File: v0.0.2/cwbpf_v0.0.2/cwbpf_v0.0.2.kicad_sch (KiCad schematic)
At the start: 9 parts, among them J1 AudioJack4, U1 PCM5102A, U2 PCM1808PWR

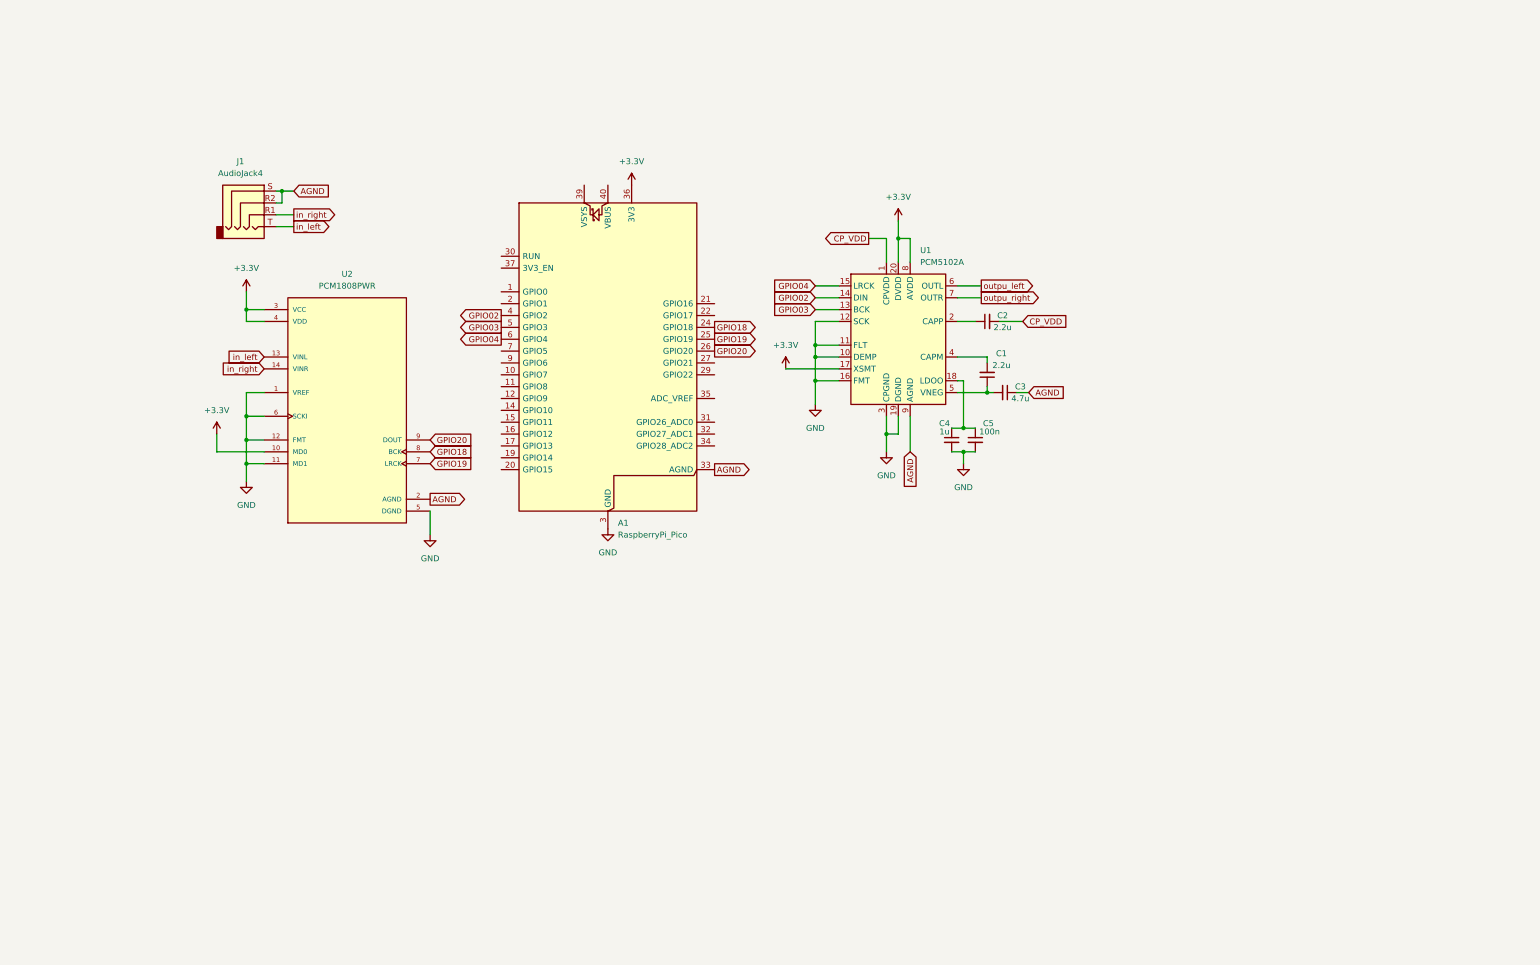
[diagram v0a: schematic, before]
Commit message: tmp
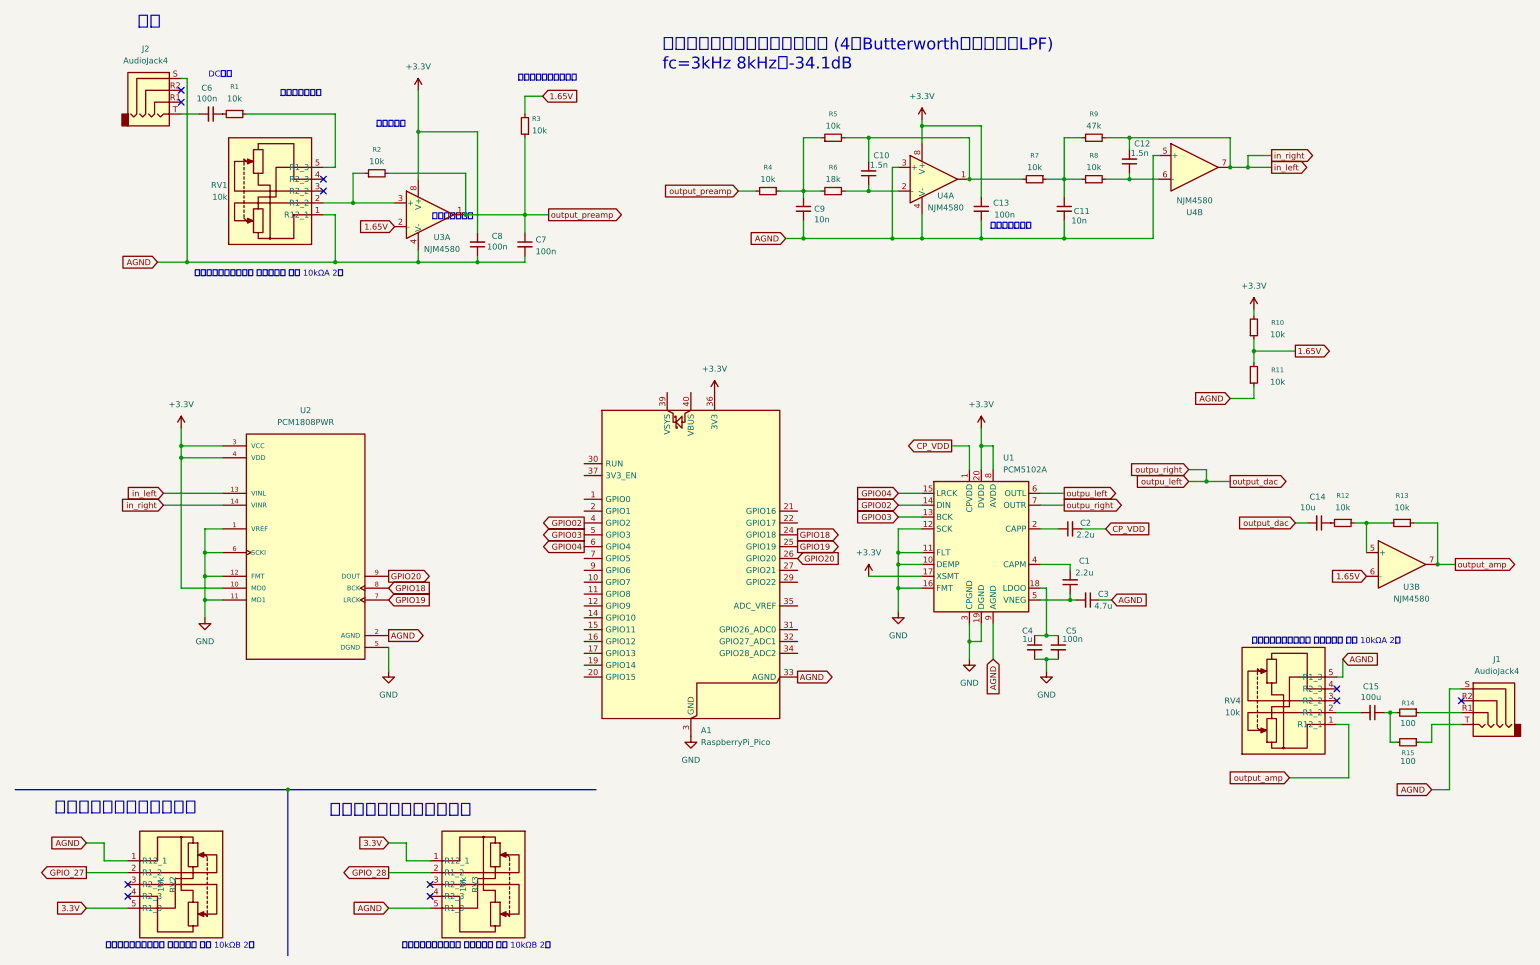
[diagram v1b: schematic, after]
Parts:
- added C10, C12: 1.5n, Capacitor_THT:C_Disc_D7.0mm_W2.5mm_P5.00mm, symbol Device:C_Small
- added C11, C9: 10n, Capacitor_THT:C_Disc_D7.0mm_W2.5mm_P5.00mm, symbol Device:C_Small
- added C13, C6, C7, C8: 100n, Capacitor_THT:C_Disc_D7.5mm_W2.5mm_P5.00mm, symbol Device:C_Small
- added C14: 10u, Capacitor_THT:CP_Radial_D5.0mm_P2.00mm, symbol Device:C_Small
- added C15: 100u, Capacitor_THT:CP_Radial_D8.0mm_P3.50mm, symbol Device:C_Small
- added J2: AudioJack4, Connector_Audio:Jack_3.5mm_PJ320E_Horizontal, symbol Connector_Audio:AudioJack4
- added R1, R10, R11, R12, R13, R2, R3, R4, R5, R7, R8: 10k, Resistor_THT:R_Axial_DIN0204_L3.6mm_D1.6mm_P5.08mm_Horizontal, symbol Device:R_Small
- added R14, R15: 100, Resistor_THT:R_Axial_DIN0204_L3.6mm_D1.6mm_P5.08mm_Horizontal, symbol Device:R_Small
- added R6: 18k, Resistor_THT:R_Axial_DIN0204_L3.6mm_D1.6mm_P5.08mm_Horizontal, symbol Device:R_Small
- added R9: 47k, Resistor_THT:R_Axial_DIN0204_L3.6mm_D1.6mm_P5.08mm_Horizontal, symbol Device:R_Small
- added RV1, RV2, RV3, RV4: 10k, Library:基板取付用ボリューム つまみ付き 薄型 10kΩ 2連, symbol Library:基板取付用ボリューム つまみ付き 薄型 2連
- added U3, U4: NJM4580, Package_SIP:SIP-8_19x3mm_P2.54mm, symbol Amplifier_Operational:NJM4580
- J1: footprint (none) -> Connector_Audio:Jack_3.5mm_PJ320E_Horizontal
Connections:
- net outpu_right is gone; now on net outpu_left: U1.7 (OUTR)
- net +3.3V: now also C13.1, C8.2, R10.2, U3.8 (V+), U4.8 (V+)
- net AGND: now also C11.2, C13.2, C7.2, C8.1, C9.2, J2.S, R11.1, RV1.1 (R12_1), RV2.1 (R12_1), RV3.5 (R1_3), RV4.5 (R1_3), U3.4 (V-), U4.3 (+), U4.4 (V-), U4.5 (+); no longer J1.R2
- net in_left: now also U2.14 (VINR), C12.2, R9.2, U4.7; no longer J1.T
- net outpu_left: now also C14.2
- net in_right: no longer names the net of J1.R1
- net in_right: now also R14.1; no longer U2.14 (VINR)
- new net: R12.1, R13.2, U3.5 (+)
- new net: J1.T, R15.1
- new net: C14.1, R12.2
- new net: C11.1, R7.1, R8.1, R9.1
- new net: C15.1, R14.2, R15.2
- new net: C15.2, RV4.2 (R1_2)
- new net: C9.1, R4.1, R5.1, R6.1
- new net: R2.1, RV1.2 (R1_2), U3.3 (+)
- new net: C10.2, R5.2, R7.2, U4.1
- new net: C6.2, J2.T
- new net: C10.1, R6.2, U4.2 (-)
- new net: C12.1, R8.2, U4.6 (-)
- new net: R1.1, RV1.5 (R1_3)
- new net: C6.1, R1.2
- new net 1.65V: R10.1, R11.2, R3.2, U3.2 (-), U3.6 (-)
- new net 3.3V: RV2.5 (R1_3), RV3.1 (R12_1)
- new net GPIO_27: RV2.2 (R1_2)
- new net GPIO_28: RV3.2 (R1_2)
- new net output_amp: R13.1, RV4.1 (R12_1), U3.7
- new net output_preamp: C7.1, R2.2, R3.1, R4.2, U3.1
- no-connect marks 0 -> 11
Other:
- note added: "DC遮断"
- note added: "アンチエイリアシングフィルタ (4次Butterworth多重帰還型LPF) fc=3kHz 8kHzで-34.1dB"
- note added: "デカップリング"
- note added: "バイアス電圧重畳回路"
- note added: "プリアンプ"
- note added: "上限周波数調整ボリューム"
- note added: "下限周波数調整ボリューム"
- note added: "入力"
- note added: "入力ゲイン調整"
- note added: "基板取付用ボリューム つまみ付き 薄型 10kΩA 2連"
- note added: "基板取付用ボリューム つまみ付き 薄型 10kΩB 2連"
- moved on the sheet: A1, C1, C2, C3, C4, C5, U1, U2
